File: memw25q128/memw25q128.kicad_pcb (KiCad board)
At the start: 2 copper layers, 76.2 x 50.8 mm, 15 parts, among them J1 STM32WORLD_BASE, U1 W25Q128JVS

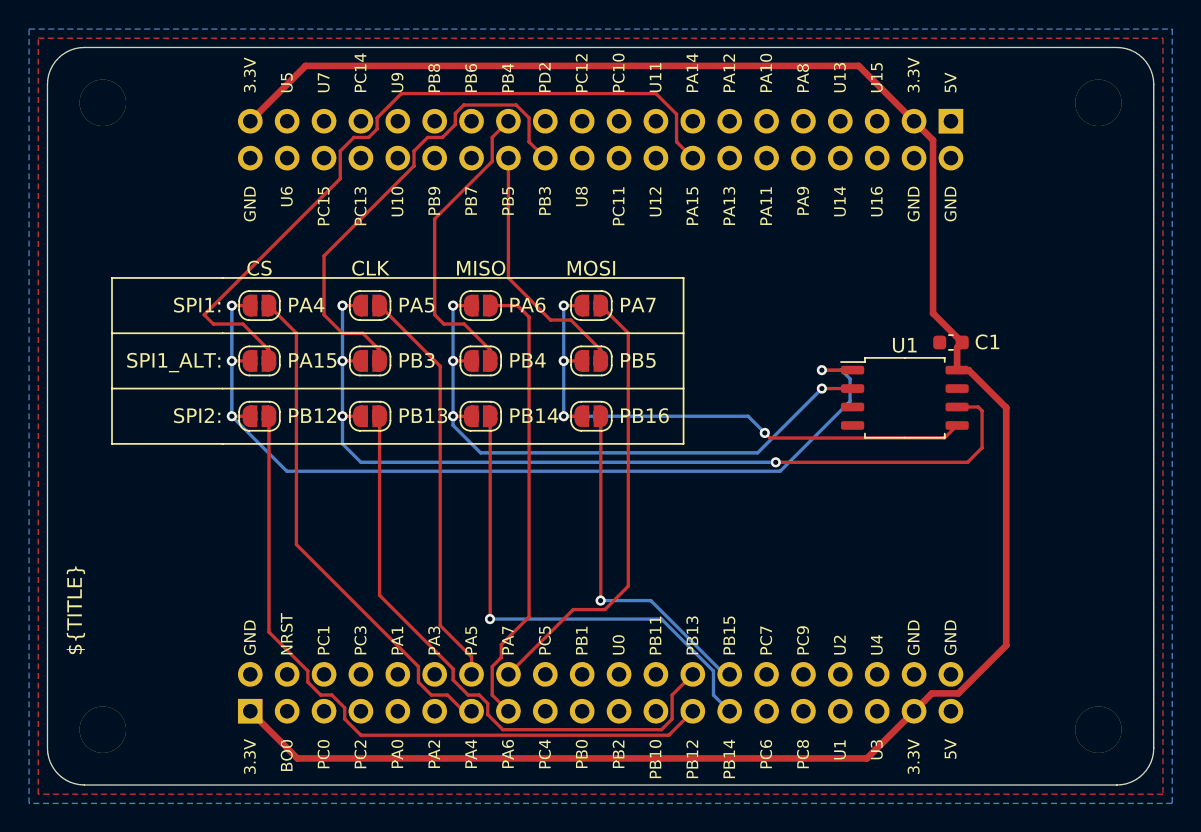
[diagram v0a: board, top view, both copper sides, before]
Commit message: Playing with ordering files
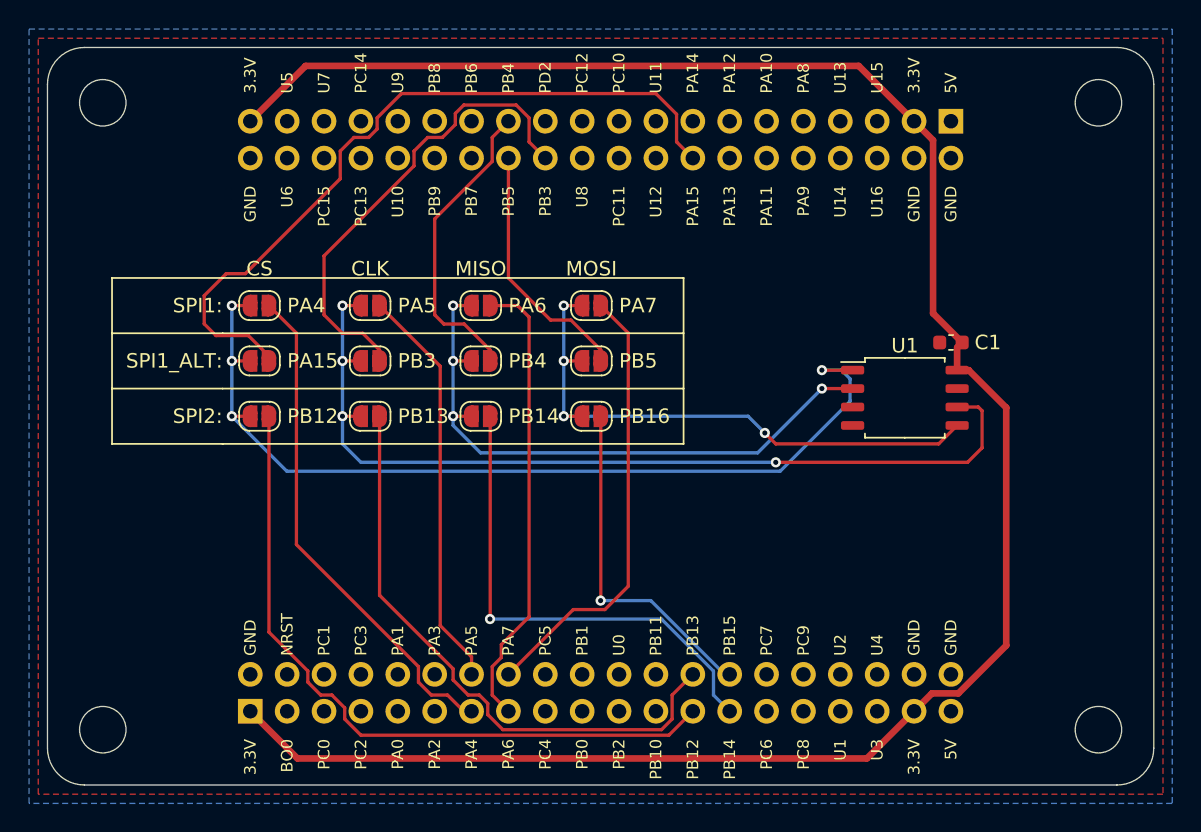
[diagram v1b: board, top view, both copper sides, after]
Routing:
- net PA15: track 50.7 -> 51.6 mm
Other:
- board text removed: "${TITLE}"
